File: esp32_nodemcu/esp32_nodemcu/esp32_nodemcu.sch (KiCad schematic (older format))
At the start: 3 parts, among them J1 Conn_01x02_Female

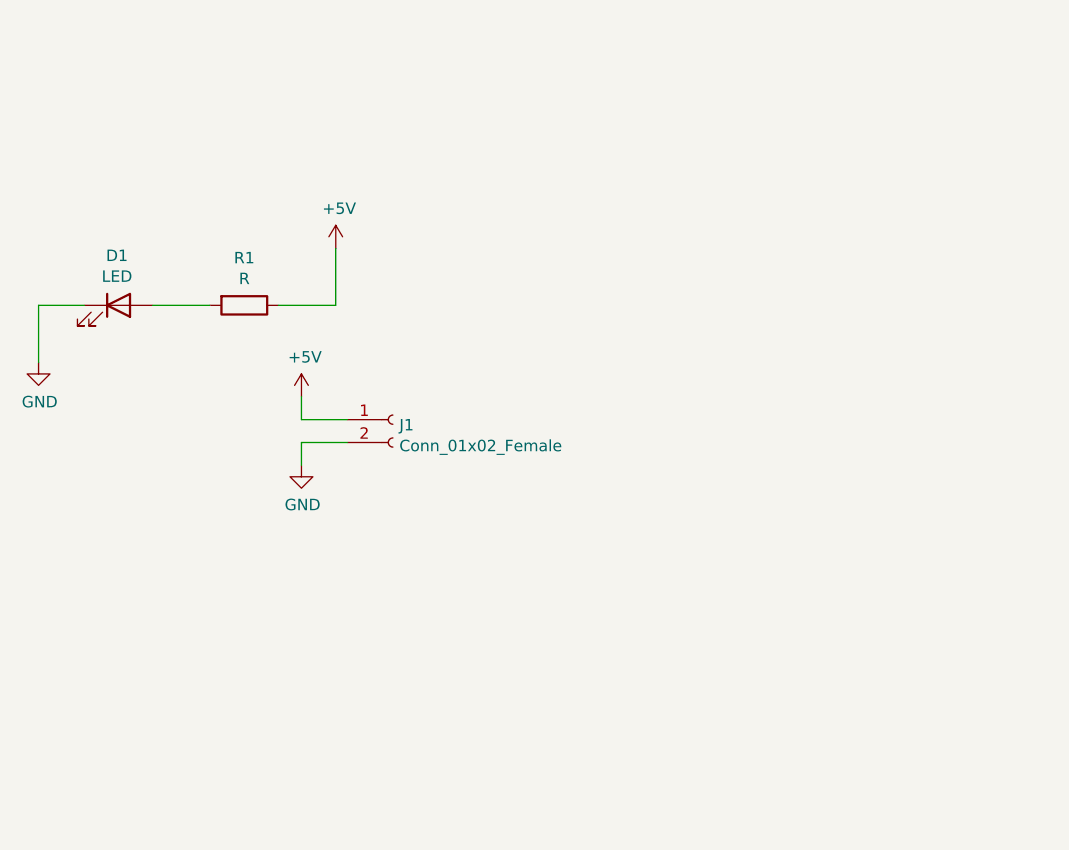
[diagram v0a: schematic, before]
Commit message: pcb update
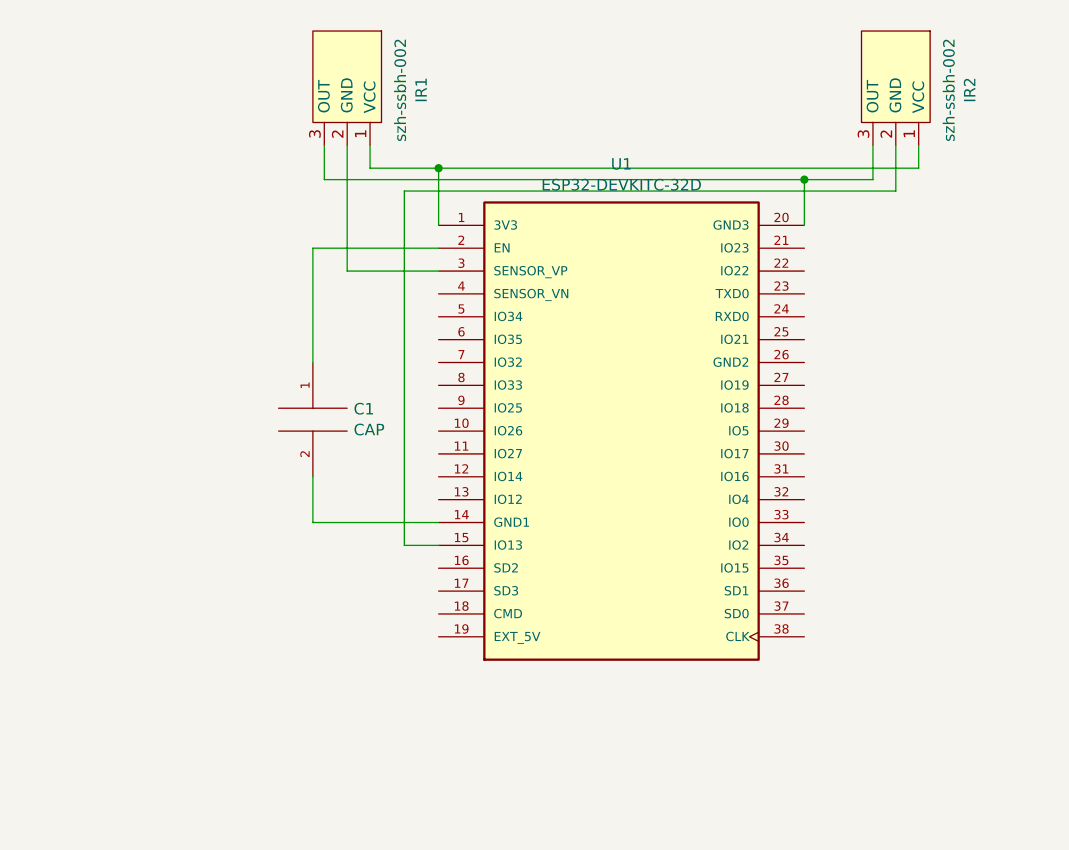
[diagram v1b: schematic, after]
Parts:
- removed D1: LED, LED_THT:LED_D3.0mm, symbol Device:LED
- removed J1: Conn_01x02_Female, Connector_Molex:Molex_KK-254_AE-6410-02A_1x02_P2.54mm_Vertical, symbol Connector:Conn_01x02_Female
- removed R1: R, Resistor_THT:R_Axial_DIN0207_L6.3mm_D2.5mm_P7.62mm_Horizontal, symbol Device:R
- added C1: CAP, Capacitor_THT:CP_Radial_D10.0mm_P5.00mm, symbol pspice:CAP
- added IR1, IR2: szh-ssbh-002, Connector_PinHeader_2.54mm:PinHeader_1x03_P2.54mm_Horizontal, symbol szh_ssbh-002:szh-ssbh-002
- added U1: ESP32-DEVKITC-32D, ESP32-DEVKITC-32D:MODULE_ESP32-DEVKITC-32D, symbol ESP32-DEVKITC-32D:ESP32-DEVKITC-32D
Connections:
- new net: IR1.1 (VCC), IR2.1 (VCC), U1.1 (3V3)
- new net: IR1.2 (GND), U1.3 (SENSOR_VP)
- new net: IR1.3 (OUT), IR2.3 (OUT), U1.20 (GND3)
- new net: IR2.2 (GND), U1.15 (IO13)
- new net: C1.1, U1.2 (EN)
- new net: C1.2, U1.14 (GND1)
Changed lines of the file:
@@
 $EndDescr
 $Comp
-L Device:LED D1
-U 1 1 6087C40F
-P 3050 2450
-F 0 "D1" H 3043 2667 50  0000 C CNN
-F 1 "LED" H 3043 2576 50  0000 C CNN
-F 2 "LED_THT:LED_D3.0mm" H 3050 2450 50  0001 C CNN
-F 3 "~" H 3050 2450 50  0001 C CNN
-	1    3050 2450
+L pspice:CAP C1
+U 1 1 6093B723
+P 3900 2950
+F 0 "C1" H 4078 2996 50  0000 L CNN
+F 1 "CAP" H 4078 2905 50  0000 L CNN
+F 2 "Capacitor_THT:CP_Radial_D10.0mm_P5.00mm" H 3900 2950 50  0001 C CNN
+F 3 "~" H 3900 2950 50  0001 C CNN
+	1    3900 2950
 	1    0    0    -1
 $EndComp
 $Comp
-L Device:R R1
-U 1 1 6087C95C
-P 3600 2450
-F 0 "R1" V 3393 2450 50  0000 C CNN
-F 1 "R" V 3484 2450 50  0000 C CNN
-F 2 "Resistor_THT:R_Axial_DIN0207_L6.3mm_D2.5mm_P7.62mm_Horizontal" V 3530 2450 50  0001 C CNN
-F 3 "~" H 3600 2450 50  0001 C CNN
-	1    3600 2450
+L szh_ssbh-002:szh-ssbh-002 IR1
+U 1 1 60939DDB
+P 4200 1350
+F 0 "IR1" H 4358 1525 50  0000 C CNN
+F 1 "szh-ssbh-002" H 4358 1434 50  0000 C CNN
+F 2 "Connector_PinHeader_2.54mm:PinHeader_1x03_P2.54mm_Horizontal" H 4100 1500 50  0001 C CNN
+F 3 "" H 4100 1500 50  0001 C CNN
+	1    4200 1350
 	0    1    1    0
 $EndComp
 $Comp
-L power:GND #PWR01
-U 1 1 6087DB88
-P 2700 2700
-F 0 "#PWR01" H 2700 2450 50  0001 C CNN
-F 1 "GND" H 2705 2527 50  0000 C CNN
-F 2 "" H 2700 2700 50  0001 C CNN
-F 3 "" H 2700 2700 50  0001 C CNN
-	1    2700 2700
-	1    0    0    -1
+L szh_ssbh-002:szh-ssbh-002 IR2
+U 1 1 6093AB17
+P 6600 1350
+F 0 "IR2" H 6758 1525 50  0000 C CNN
+F 1 "szh-ssbh-002" H 6758 1434 50  0000 C CNN
+F 2 "Connector_PinHeader_2.54mm:PinHeader_1x03_P2.54mm_Horizontal" H 6500 1500 50  0001 C CNN
+F 3 "" H 6500 1500 50  0001 C CNN
+	1    6600 1350
+	0    1    1    0
 $EndComp
+Wire Wire Line
+	4450 2200 3900 2200
+Wire Wire Line
+	3900 2200 3900 2700
+Wire Wire Line
+	3900 3200 3900 3400
+Wire Wire Line
+	3900 3400 4450 3400
+Wire Wire Line
+	4450 1850 6550 1850
+Wire Wire Line
+	6550 1850 6550 1750
+Connection ~ 4450 1850
+Wire Wire Line
+	4450 1850 4450 2100
+Wire Wire Line
+	4450 1850 4150 1850
+Wire Wire Line
+	4150 1850 4150 1750
 $Comp
-L power:+5V #PWR04
-U 1 1 6087E174
-P 4000 2200
-F 0 "#PWR04" H 4000 2050 50  0001 C CNN
-F 1 "+5V" H 4015 2373 50  0000 C CNN
-F 2 "" H 4000 2200 50  0001 C CNN
-F 3 "" H 4000 2200 50  0001 C CNN
-	1    4000 2200
+L ESP32-DEVKITC-32D:ESP32-DEVKITC-32D U1
+U 1 1 609438B2
+P 5250 3000
+F 0 "U1" H 5250 4167 50  0000 C CNN
+F 1 "ESP32-DEVKITC-32D" H 5250 4076 50  0000 C CNN
+F 2 "ESP32-DEVKITC-32D:MODULE_ESP32-DEVKITC-32D" H 5250 3000 50  0001 L BNN
+F 3 "" H 5250 3000 50  0001 L BNN
+F 4 "Espressif Systems" H 5250 3000 50  0001 L BNN "MANUFACTURER"
+F 5 "4" H 5250 3000 50  0001 L BNN "PARTREV"
+	1    5250 3000
 	1    0    0    -1
 $EndComp
 Wire Wire Line
-	4000 2200 4000 2450
+	6050 2100 6050 1900
 Wire Wire Line
-	3750 2450 4000 2450
+	6050 1900 6350 1900
 Wire Wire Line
-	3200 2450 3450 2450
+	6350 1900 6350 1750
 Wire Wire Line
-	2700 2450 2900 2450
+	6050 1900 3950 1900
 Wire Wire Line
-	2700 2450 2700 2700
-$Comp
-L Connector:Conn_01x02_Female J1
-U 1 1 6087FCFA
-P 4250 2950
-F 0 "J1" H 4278 2926 50  0000 L CNN
-F 1 "Conn_01x02_Female" H 4278 2835 50  0000 L CNN
-F 2 "Connector_Molex:Molex_KK-254_AE-6410-02A_1x02_P2.54mm_Vertical" H 4250 2950 50  0001 C CNN
-F 3 "~" H 4250 2950 50  0001 C CNN
-	1    4250 2950
-	1    0    0    -1
-$EndComp
-$Comp
-L power:+5V #PWR02
-U 1 1 6088086A
-P 3850 2850
-F 0 "#PWR02" H 3850 2700 50  0001 C CNN
-F 1 "+5V" H 3865 3023 50  0000 C CNN
-F 2 "" H 3850 2850 50  0001 C CNN
-F 3 "" H 3850 2850 50  0001 C CNN
-	1    3850 2850
-	1    0    0    -1
-$EndComp
-$Comp
-L power:GND #PWR03
-U 1 1 60880F82
-P 3850 3150
-F 0 "#PWR03" H 3850 2900 50  0001 C CNN
-F 1 "GND" H 3855 2977 50  0000 C CNN
-F 2 "" H 3850 3150 50  0001 C CNN
-F 3 "" H 3850 3150 50  0001 C CNN
-	1    3850 3150
-	1    0    0    -1
-$EndComp
+	3950 1900 3950 1750
+Connection ~ 6050 1900
 Wire Wire Line
-	3850 2850 3850 2950
+	4050 1750 4050 2300
 Wire Wire Line
-	3850 2950 4050 2950
+	4050 2300 4450 2300
 Wire Wire Line
-	3850 3150 3850 3050
+	6450 1750 6450 1950
 Wire Wire Line
-	3850 3050 4050 3050
+	6450 1950 4300 1950
+Wire Wire Line
+	4300 1950 4300 3500
+Wire Wire Line
+	4300 3500 4450 3500
 $EndSCHEMATC

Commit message: pcb update
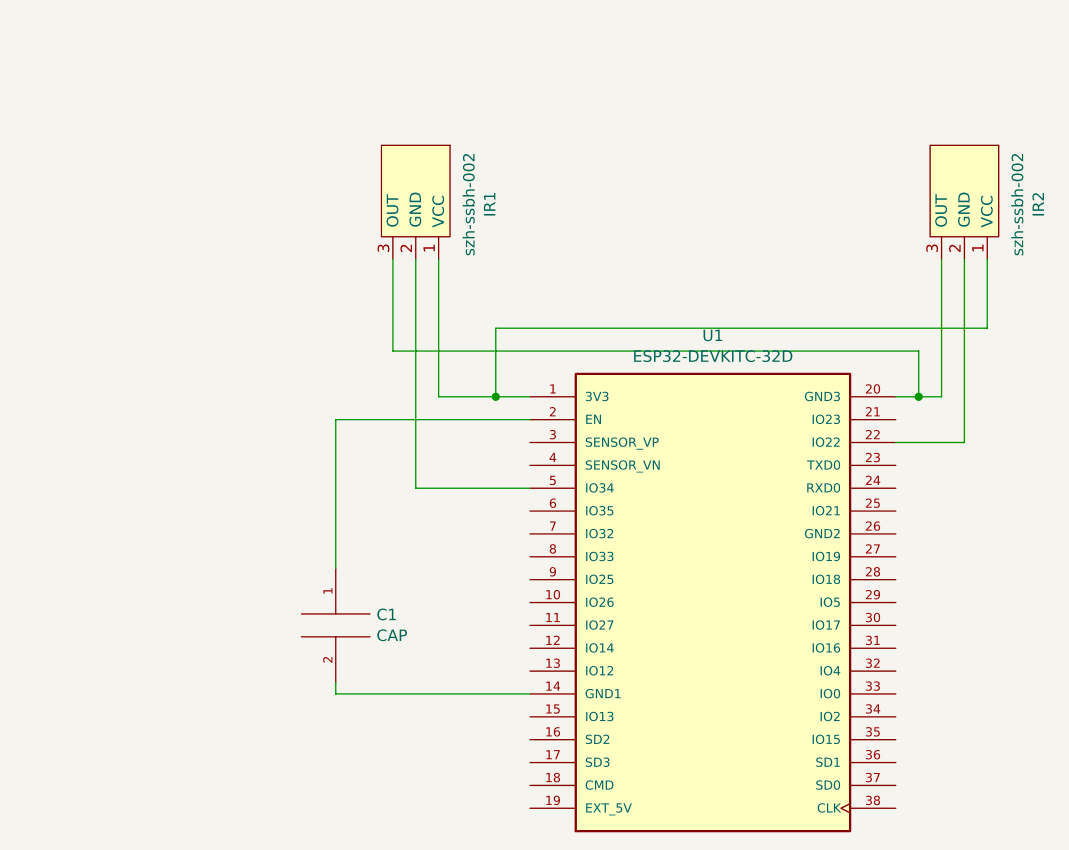
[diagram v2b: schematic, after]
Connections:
- net at IR1.2 (GND): now also U1.5 (IO34); no longer U1.3 (SENSOR_VP)
- net at IR2.2 (GND): now also U1.22 (IO22); no longer U1.15 (IO13)
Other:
- moved on the sheet: C1, IR1, IR2, U1
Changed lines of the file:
@@
 $EndDescr
-$Comp
-L pspice:CAP C1
-U 1 1 6093B723
-P 3900 2950
-F 0 "C1" H 4078 2996 50  0000 L CNN
-F 1 "CAP" H 4078 2905 50  0000 L CNN
-F 2 "Capacitor_THT:CP_Radial_D10.0mm_P5.00mm" H 3900 2950 50  0001 C CNN
-F 3 "~" H 3900 2950 50  0001 C CNN
-	1    3900 2950
-	1    0    0    -1
-$EndComp
 $Comp
 L szh_ssbh-002:szh-ssbh-002 IR1
 U 1 1 60939DDB
-P 4200 1350
-F 0 "IR1" H 4358 1525 50  0000 C CNN
-F 1 "szh-ssbh-002" H 4358 1434 50  0000 C CNN
-F 2 "Connector_PinHeader_2.54mm:PinHeader_1x03_P2.54mm_Horizontal" H 4100 1500 50  0001 C CNN
-F 3 "" H 4100 1500 50  0001 C CNN
-	1    4200 1350
+P 4500 1850
+F 0 "IR1" H 4658 2025 50  0000 C CNN
+F 1 "szh-ssbh-002" H 4658 1934 50  0000 C CNN
+F 2 "Connector_PinHeader_2.54mm:PinHeader_1x03_P2.54mm_Horizontal" H 4400 2000 50  0001 C CNN
+F 3 "" H 4400 2000 50  0001 C CNN
+	1    4500 1850
 	0    1    1    0
 $EndComp
@@
 L szh_ssbh-002:szh-ssbh-002 IR2
 U 1 1 6093AB17
-P 6600 1350
-F 0 "IR2" H 6758 1525 50  0000 C CNN
-F 1 "szh-ssbh-002" H 6758 1434 50  0000 C CNN
-F 2 "Connector_PinHeader_2.54mm:PinHeader_1x03_P2.54mm_Horizontal" H 6500 1500 50  0001 C CNN
-F 3 "" H 6500 1500 50  0001 C CNN
-	1    6600 1350
+P 6900 1850
+F 0 "IR2" H 7058 2025 50  0000 C CNN
+F 1 "szh-ssbh-002" H 7058 1934 50  0000 C CNN
+F 2 "Connector_PinHeader_2.54mm:PinHeader_1x03_P2.54mm_Horizontal" H 6800 2000 50  0001 C CNN
+F 3 "" H 6800 2000 50  0001 C CNN
+	1    6900 1850
 	0    1    1    0
 $EndComp
-Wire Wire Line
-	4450 2200 3900 2200
-Wire Wire Line
-	3900 2200 3900 2700
-Wire Wire Line
-	3900 3200 3900 3400
-Wire Wire Line
-	3900 3400 4450 3400
-Wire Wire Line
-	4450 1850 6550 1850
-Wire Wire Line
-	6550 1850 6550 1750
-Connection ~ 4450 1850
-Wire Wire Line
-	4450 1850 4450 2100
-Wire Wire Line
-	4450 1850 4150 1850
-Wire Wire Line
-	4150 1850 4150 1750
+$Comp
+L pspice:CAP C1
+U 1 1 6093B723
+P 4000 3850
+F 0 "C1" H 4178 3896 50  0000 L CNN
+F 1 "CAP" H 4178 3805 50  0000 L CNN
+F 2 "Capacitor_THT:CP_Radial_D10.0mm_P5.00mm" H 4000 3850 50  0001 C CNN
+F 3 "~" H 4000 3850 50  0001 C CNN
+	1    4000 3850
+	1    0    0    -1
+$EndComp
 $Comp
 L ESP32-DEVKITC-32D:ESP32-DEVKITC-32D U1
 U 1 1 609438B2
-P 5250 3000
-F 0 "U1" H 5250 4167 50  0000 C CNN
-F 1 "ESP32-DEVKITC-32D" H 5250 4076 50  0000 C CNN
-F 2 "ESP32-DEVKITC-32D:MODULE_ESP32-DEVKITC-32D" H 5250 3000 50  0001 L BNN
-F 3 "" H 5250 3000 50  0001 L BNN
-F 4 "Espressif Systems" H 5250 3000 50  0001 L BNN "MANUFACTURER"
-F 5 "4" H 5250 3000 50  0001 L BNN "PARTREV"
-	1    5250 3000
+P 5650 3750
+F 0 "U1" H 5650 4917 50  0000 C CNN
+F 1 "ESP32-DEVKITC-32D" H 5650 4826 50  0000 C CNN
+F 2 "ESP32-DEVKITC-32D:MODULE_ESP32-DEVKITC-32D" H 5650 3750 50  0001 L BNN
+F 3 "" H 5650 3750 50  0001 L BNN
+F 4 "Espressif Systems" H 5650 3750 50  0001 L BNN "MANUFACTURER"
+F 5 "4" H 5650 3750 50  0001 L BNN "PARTREV"
+	1    5650 3750
 	1    0    0    -1
 $EndComp
 Wire Wire Line
-	6050 2100 6050 1900
+	4850 2950 4000 2950
 Wire Wire Line
-	6050 1900 6350 1900
+	4000 2950 4000 3600
 Wire Wire Line
-	6350 1900 6350 1750
+	4000 4100 4000 4150
 Wire Wire Line
-	6050 1900 3950 1900
+	4000 4150 4850 4150
 Wire Wire Line
-	3950 1900 3950 1750
-Connection ~ 6050 1900
+	6650 2250 6650 2850
 Wire Wire Line
-	4050 1750 4050 2300
+	6650 2850 6550 2850
 Wire Wire Line
-	4050 2300 4450 2300
+	6850 2250 6850 2550
 Wire Wire Line
-	6450 1750 6450 1950
+	6850 2550 4700 2550
 Wire Wire Line
-	6450 1950 4300 1950
+	4700 2550 4700 2850
 Wire Wire Line
-	4300 1950 4300 3500
+	4700 2850 4850 2850
 Wire Wire Line
-	4300 3500 4450 3500
+	4250 2250 4250 2650
+Wire Wire Line
+	4250 2650 6550 2650
+Wire Wire Line
+	6550 2650 6550 2850
+Connection ~ 6550 2850
+Wire Wire Line
+	6550 2850 6450 2850
+Wire Wire Line
+	4450 2250 4450 2850
+Wire Wire Line
+	4450 2850 4700 2850
+Connection ~ 4700 2850
+Wire Wire Line
+	6750 2250 6750 3050
+Wire Wire Line
+	6750 3050 6450 3050
+Wire Wire Line
+	4350 2250 4350 3250
+Wire Wire Line
+	4350 3250 4850 3250
 $EndSCHEMATC
